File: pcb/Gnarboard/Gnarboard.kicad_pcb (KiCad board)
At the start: 2 copper layers, 157.5 x 124.5 mm, 106 parts, among them J1 Screw_Terminal_01x08, J2 Screw_Terminal_01x08, J3 Screw_Terminal_01x12, J4 Screw_Terminal_01x12, Q1 MMBT5551L, Q10 IRF4905, Q11 MMBT5551L, Q12 IRF4905, Q13 MMBT5551L, Q14 IRF4905, Q15 MMBT5551L, Q16 IRF4905, Q2 IRF4905, Q3 MMBT5551L, Q4 IRF4905, Q5 MMBT5551L, Q6 IRF4905, Q7 MMBT5551L, Q8 IRF4905, Q9 MMBT5551L, U10 ACS725xLCTR-20AU, U11 ACS725xLCTR-20AU, U12 ACS725xLCTR-20AU, U2 MCP3208, U4 D24V5F3, U5 ACS725xLCTR-20AU, U6 ACS725xLCTR-20AU, U7 ACS725xLCTR-20AU, U8 ACS725xLCTR-20AU, U9 ACS725xLCTR-20AU

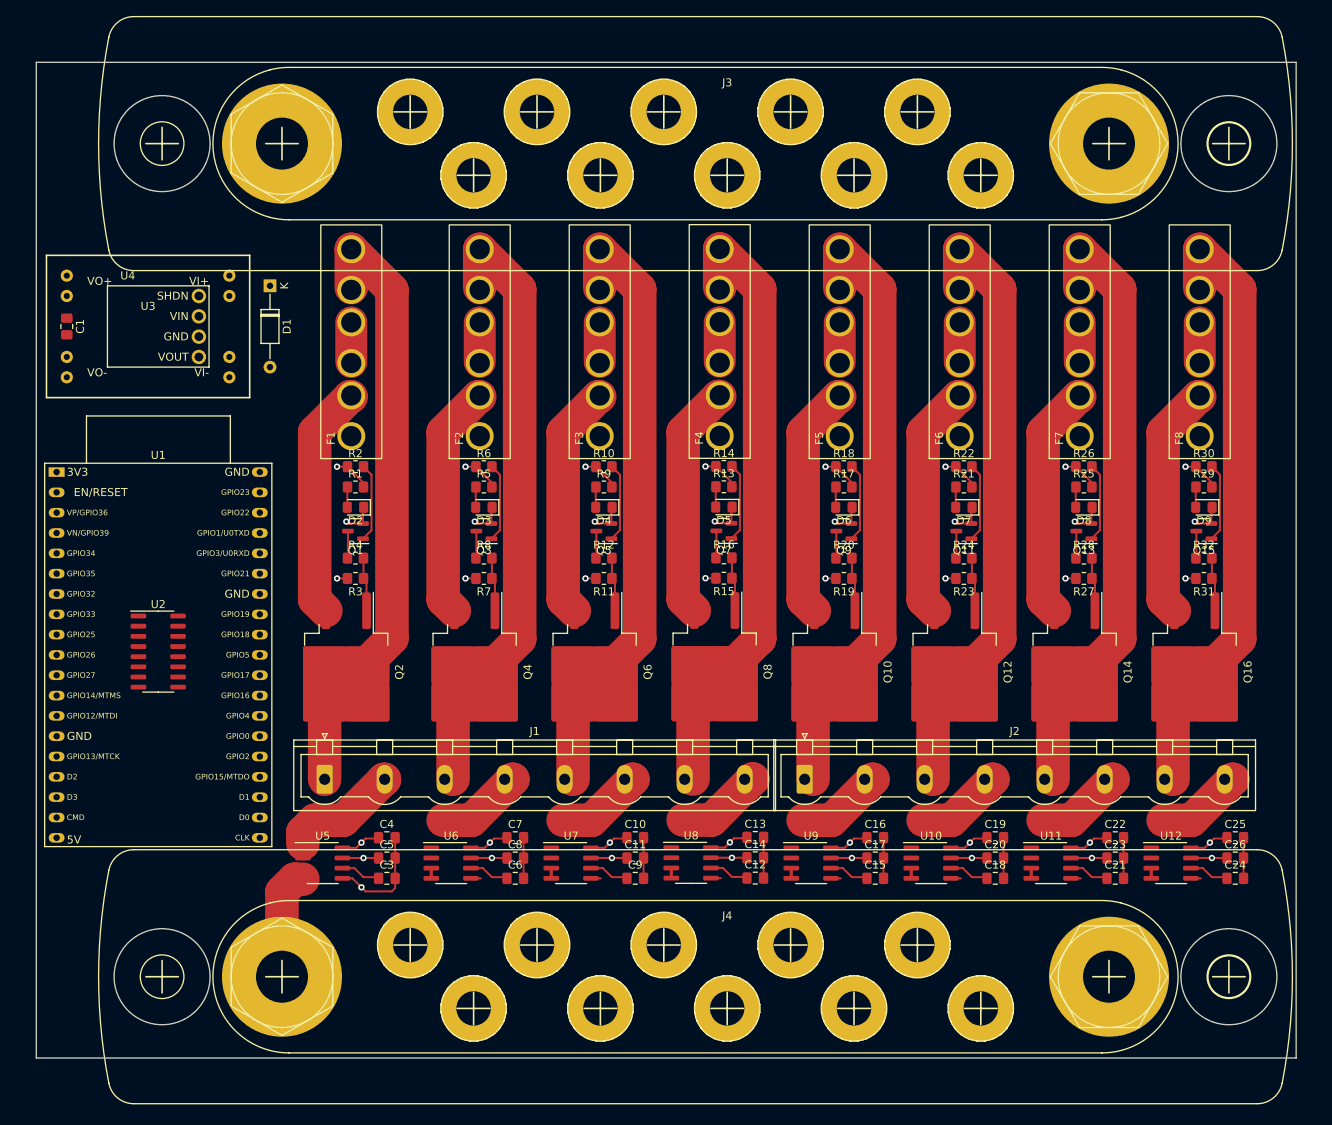
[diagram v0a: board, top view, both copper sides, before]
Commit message: board mostly laid out.
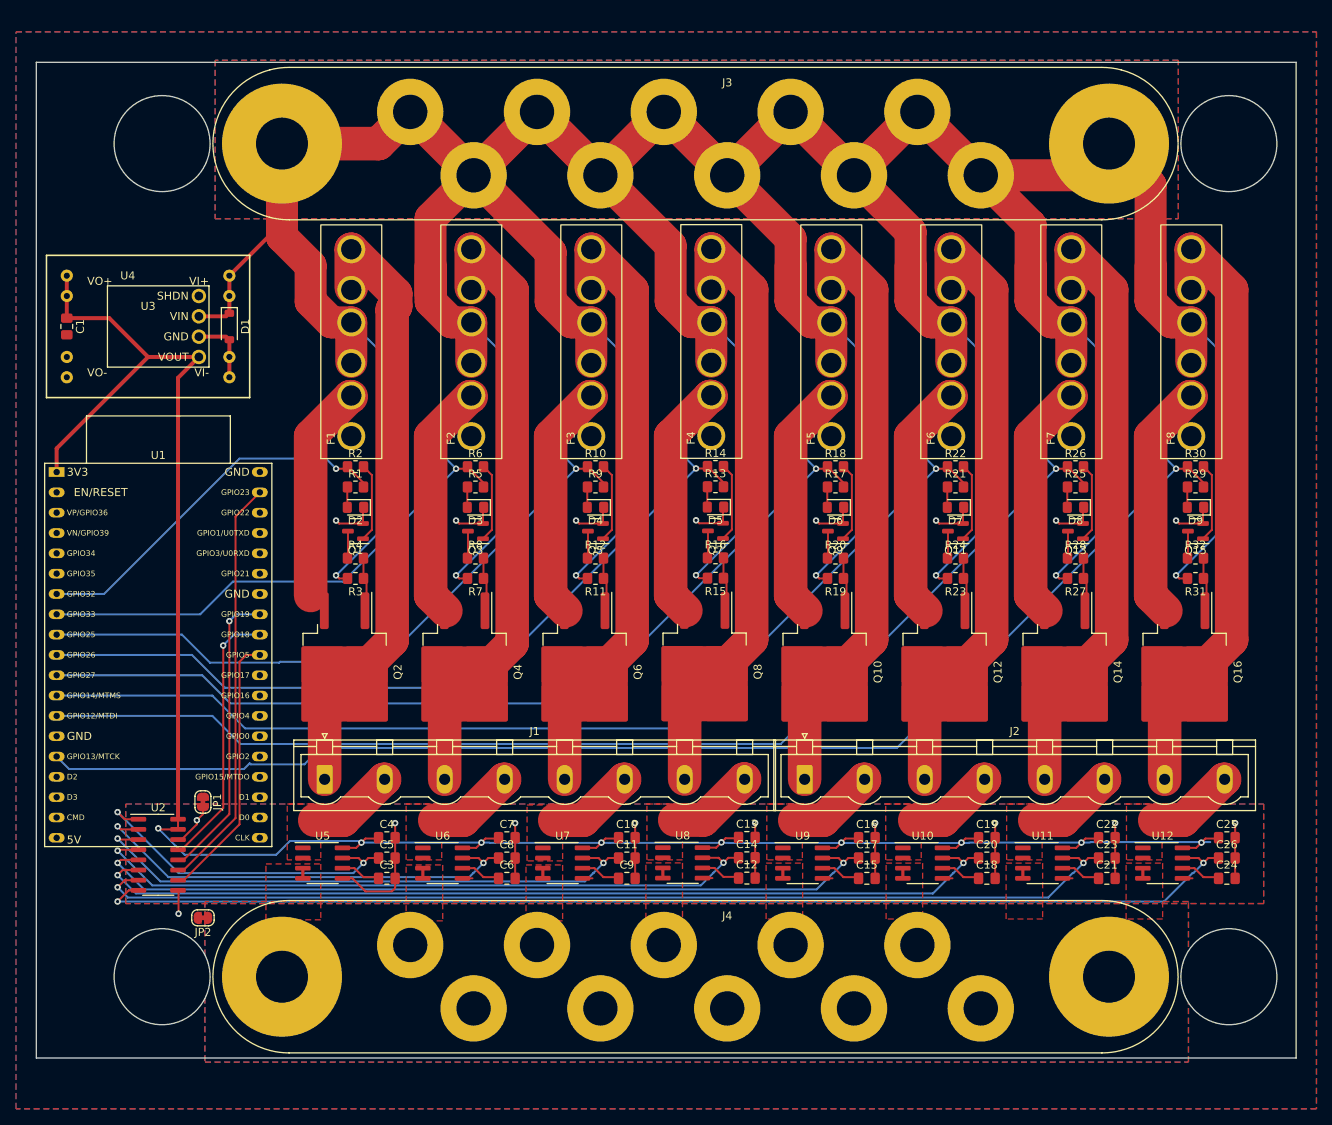
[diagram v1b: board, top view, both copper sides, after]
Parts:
- added JP1: SolderJumper_2_Bridged, Jumper:SolderJumper-2_P1.3mm_Bridged_RoundedPad1.0x1.5mm, F.Cu at (81.8, 121.7)
- added JP2: SolderJumper_2_Bridged, Jumper:SolderJumper-2_P1.3mm_Bridged_RoundedPad1.0x1.5mm, F.Cu at (81.8, 136.1)
- D1: footprint Diode_THT:D_DO-35_SOD27_P10.16mm_Horizontal -> Diode_SMD:D_SOD-123
- moved U2 25.4 mm to (76.2, 128.3)
- moved D1 7.18 mm to (85.1, 62.2)
- moved Q10 1.25 mm to (159.5, 105.4)
- moved Q12 1.25 mm to (174.5, 105.4)
- moved Q14 1.25 mm to (189.5, 105.4)
- moved Q16 1.25 mm to (204.5, 105.4)
- moved Q4 1.25 mm to (114.5, 105.4)
- moved Q6 1.25 mm to (129.5, 105.4)
- moved Q8 1.25 mm to (144.5, 105.4)
- moved C10 1.06 mm to (134.8, 126.1)
- moved C11 1.06 mm to (134.8, 128.7)
- moved C12 1.06 mm to (149.8, 131.2)
- moved C13 1.06 mm to (149.8, 126.1)
- moved C14 1.06 mm to (149.8, 128.6)
- moved C15 1.06 mm to (164.8, 131.2)
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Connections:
- D1 pad 2: GNDPWR -> GNDD
- U3 pad 4: GNDA -> GNDD
- U3 pad 5: GNDPWR -> GNDD
- U3 pad 6: GNDPWR -> GNDD
- U4 pad 3: +24V -> GNDD
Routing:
- net +24V: track 49.9 -> 719.0 mm
- net +3.3V: track 40.3 -> 280.2 mm, vias 8 -> 9
- net /PWM7: track 4.67 -> 162.4 mm
- net /PWM6: track 4.67 -> 146.8 mm
- net /ADC7: track 4.51 -> 145.9 mm, vias 1 -> 2
- net /PWM5: track 4.67 -> 131.2 mm
- net /ADC6: track 4.51 -> 131.0 mm, vias 1 -> 2
- net /ADC5: track 4.51 -> 116.2 mm, vias 1 -> 2
- net /PWM4: track 4.67 -> 114.7 mm
- net /ADC4: track 4.51 -> 101.2 mm, vias 1 -> 2
- net /PWM3: track 4.67 -> 99.1 mm
- net /ADC3: track 4.51 -> 86.4 mm, vias 1 -> 2
- net /PWM2: track 4.67 -> 82.6 mm
- net /ADC2: track 4.51 -> 71.6 mm, vias 1 -> 2
- net /PWM1: track 4.67 -> 63.6 mm
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- added copper zone on B.Cu, net +24V
- added copper zone on F.Cu, net +24V
- added copper zone on F.Cu, net /CH-0
- added copper zone on F.Cu, net /CH-1
- added copper zone on F.Cu, net /CH-2
- added copper zone on F.Cu, net /CH-3
- added copper zone on F.Cu, net /CH-4
- added copper zone on F.Cu, net /CH-5
- added copper zone on F.Cu, net /CH-6
- added copper zone on F.Cu, net /CH-7
- added copper zone on B.Cu, net GNDA
- added copper zone on F.Cu, net GNDA
- added copper zone on B.Cu, net GNDD
- added copper zone on F.Cu, net GNDD
- added copper zone on B.Cu, net GNDPWR
- added copper zone on F.Cu, net GNDPWR
